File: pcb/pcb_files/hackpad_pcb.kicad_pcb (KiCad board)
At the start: 2 copper layers, 84 x 66 mm, 15 parts, among them SW1 SW_Push, SW2 SW_Push, SW3 SW_Push, SW4 SW_Push, SW5 SW_Push, SW6 SW_Push, SW7 RotaryEncoder_Switch, U1 MOUDLE-SEEEDUINO-XIAO, U2 ER_OLEDM0.91_1x-I2C

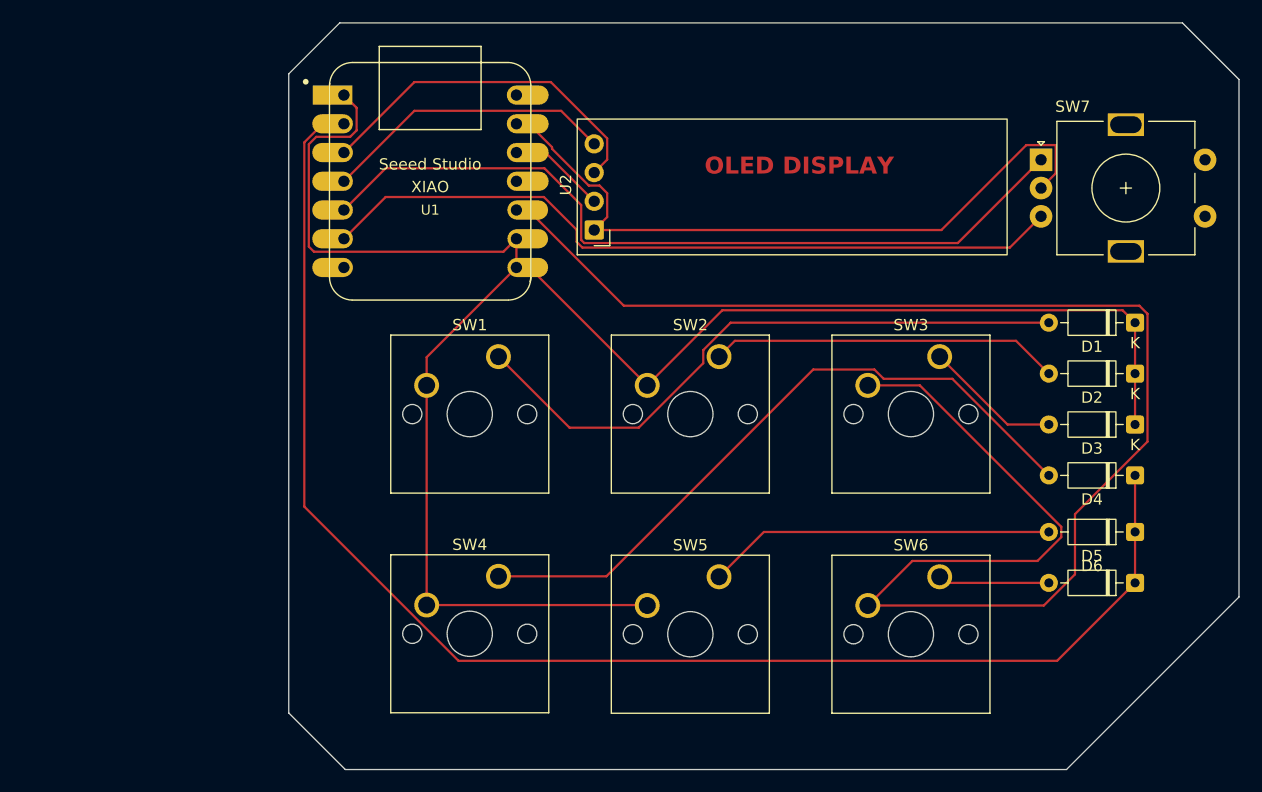
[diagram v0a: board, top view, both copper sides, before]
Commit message: Updated the PCB
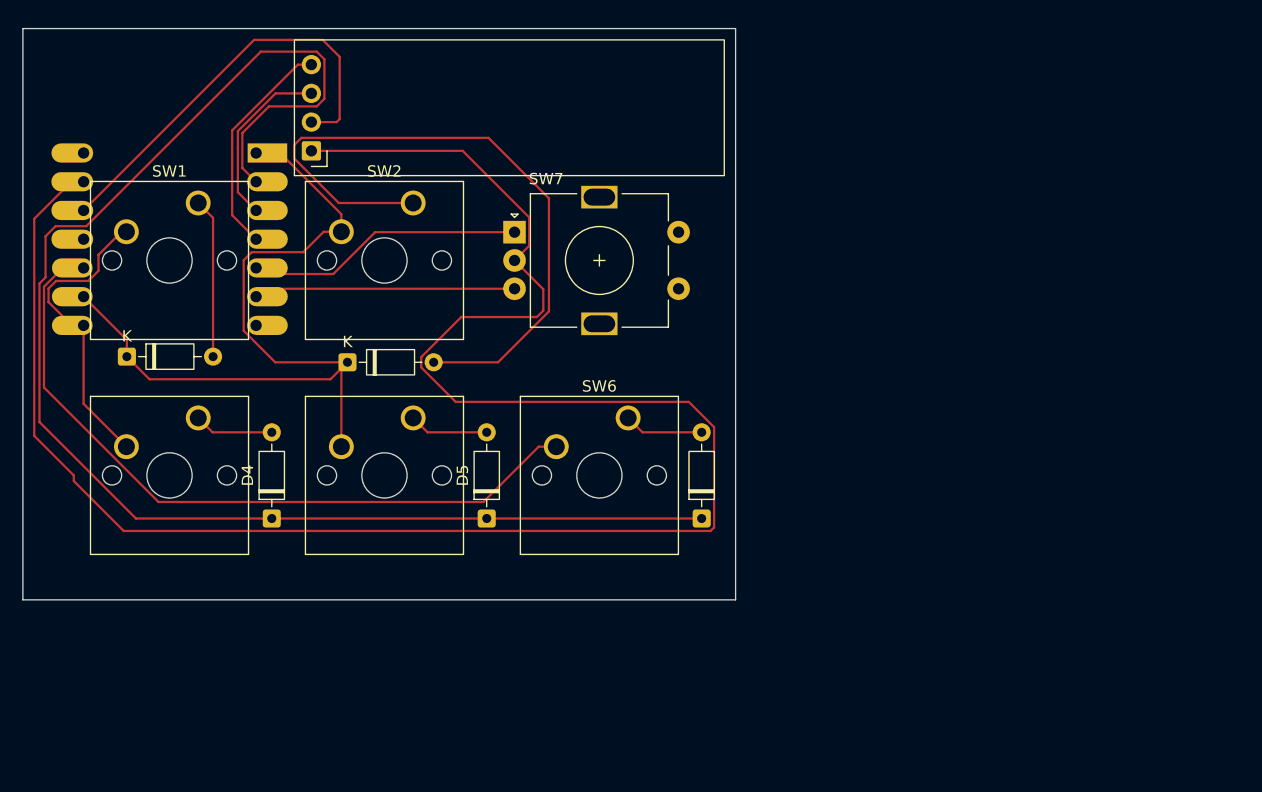
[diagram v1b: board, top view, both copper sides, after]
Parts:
- removed D3: 1N4148, Diode_THT:D_DO-35_SOD27_P7.62mm_Horizontal
- removed SW3: SW_Push, Button_Switch_Keyboard:SW_Cherry_MX_1.00u_PCB
- U1: moved to B.Cu
- moved D1 89.2 mm to (62.2, 95.0), turned to 0 degrees
- moved D4 76.4 mm to (75.0, 109.3), turned to 90 degrees
- moved D2 69.6 mm to (81.7, 95.5), turned to 0 degrees
- moved D5 57.3 mm to (94.0, 109.3), turned to 90 degrees
- moved SW7 47.0 mm to (96.5, 84.0)
- moved D6 38.7 mm to (113.0, 109.3), turned to 90 degrees
- moved SW6 30.9 mm to (106.5, 100.4)
- moved SW5 30.5 mm to (87.5, 100.4)
- moved SW2 30.3 mm to (87.5, 81.4)
- moved SW4 30.0 mm to (68.5, 100.4)
- moved SW1 29.8 mm to (68.5, 81.4)
- moved U2 26.0 mm to (78.5, 76.8)
- moved U1 23.6 mm to (66.0, 84.6), turned to 180 degrees
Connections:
- SW1 pad 2: Col_1 -> Col_2
- SW4 pad 2: Col_1 -> Col_2
- U1 pad 8: Col_1 -> Col_2
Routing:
- net GND: track 62.6 -> 170.8 mm
- net Col_1: track 163.3 -> 73.1 mm
- net Col_0: track 148.1 -> 64.6 mm
- net Net-(D4-A): track 60.1 -> 7.03 mm
- net A: track 72.3 -> 24.6 mm
- net B: track 66.8 -> 23.1 mm
- net Net-(D1-A): track 55.8 -> 14.1 mm
- net Net-(D2-A): track 30.9 -> 60.4 mm
- net 3V3: track 8.66 -> 37.6 mm
- net Col_2: track 0.00 -> 27.9 mm
- net Net-(D5-A): track 30.8 -> 7.03 mm
- net SCL: track 31.4 -> 15.6 mm
- net Net-(D3-A): track 12.1 -> 0.00 mm
- net SDA: track 25.9 -> 19.9 mm
- net Net-(D6-A): track 9.87 -> 7.03 mm
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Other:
- board size 84 x 66 mm -> 63 x 50.5 mm
- board text removed: "D6"
- board text removed: "OLED DISPLAY"
